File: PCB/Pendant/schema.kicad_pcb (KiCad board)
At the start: 2 copper layers, 5 parts

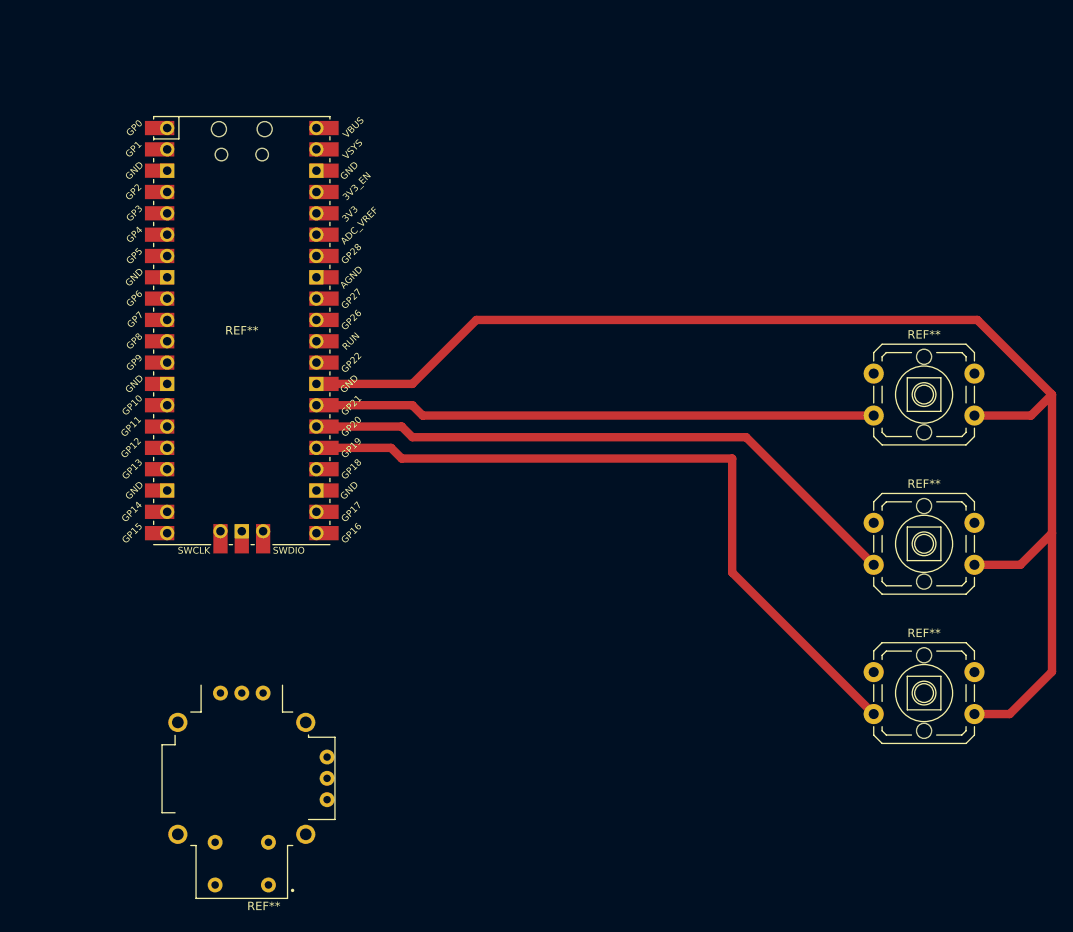
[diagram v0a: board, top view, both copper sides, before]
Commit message: PR_Březen
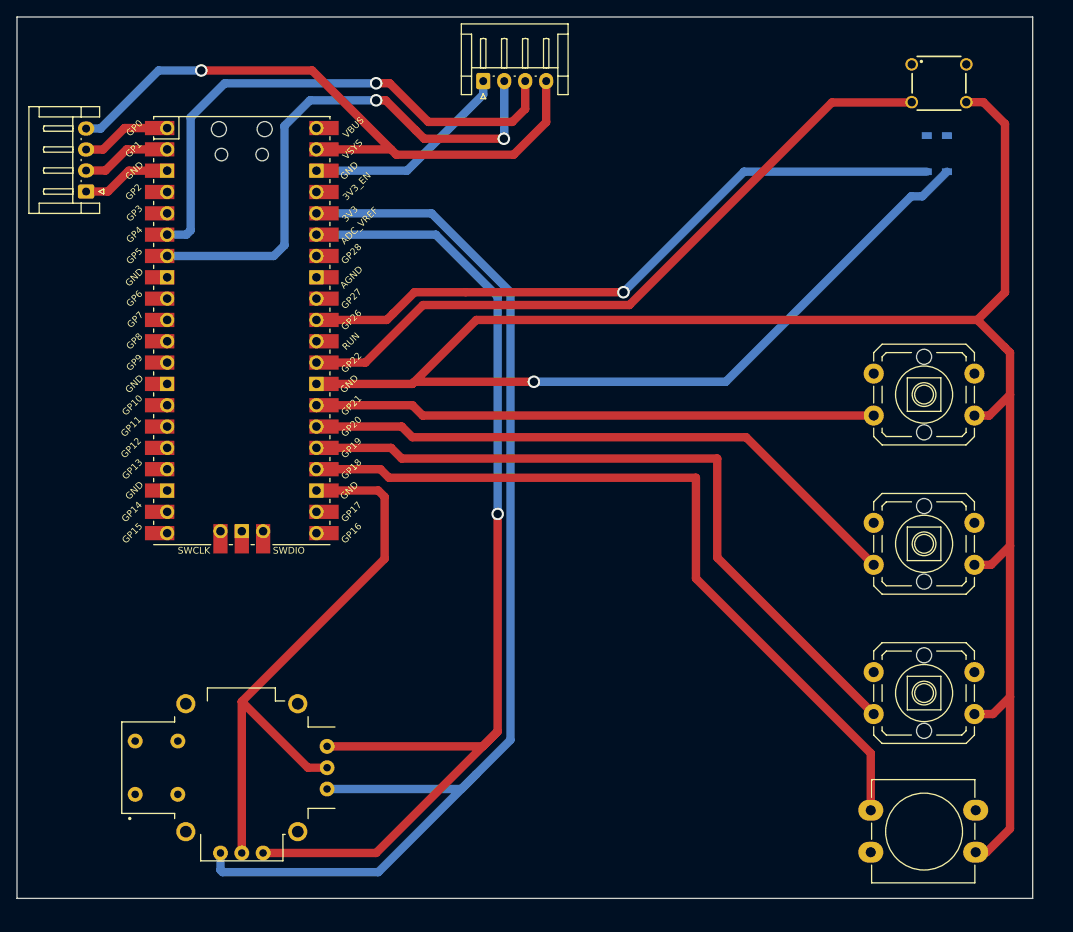
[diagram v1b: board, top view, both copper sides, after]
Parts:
- added REF**: 4301X60437X6, 4301X60437X6, F.Cu at (227.8, 56.9)
- added REF**: Detector Switch, MajLibrary:Detector Switch, B.Cu at (227.6, 65.3)
- added REF**: SW_PUSH-12mm_Wuerth-430476085716, Button_Switch_THT:SW_PUSH-12mm_Wuerth-430476085716, F.Cu at (219.7, 143.5)
- added REF**: JST_EH_S4B-EH_1x04_P2.50mm_Horizontal, Connector_JST:JST_EH_S4B-EH_1x04_P2.50mm_Horizontal, F.Cu at (126.2, 69.8)
- added REF**: JST_EH_S4B-EH_1x04_P2.50mm_Horizontal, Connector_JST:JST_EH_S4B-EH_1x04_P2.50mm_Horizontal, F.Cu at (173.5, 56.6)
- moved REF** 1.27 mm to (144.8, 138.4), turned to 90 degrees
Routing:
- net (no net): track 387.5 -> 1361.9 mm, vias 0 -> 7
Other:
- board outline added: 121 x 105 mm
